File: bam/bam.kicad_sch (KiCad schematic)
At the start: 18 parts, among them J1 battery, Q1 VP3203N3-G, Q2 PN2222A, SW1 pwr, SW2 next, SW3 play/pause, U1 NE555P

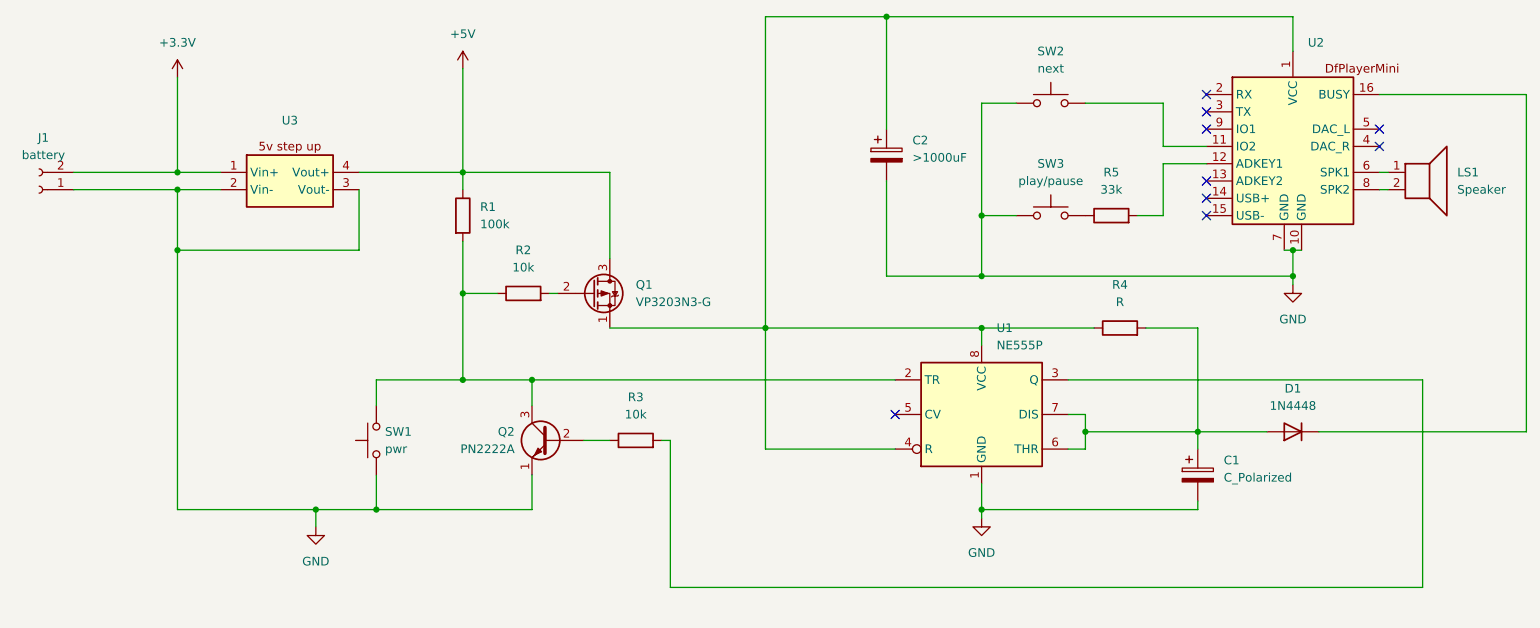
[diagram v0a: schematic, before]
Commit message: true latch
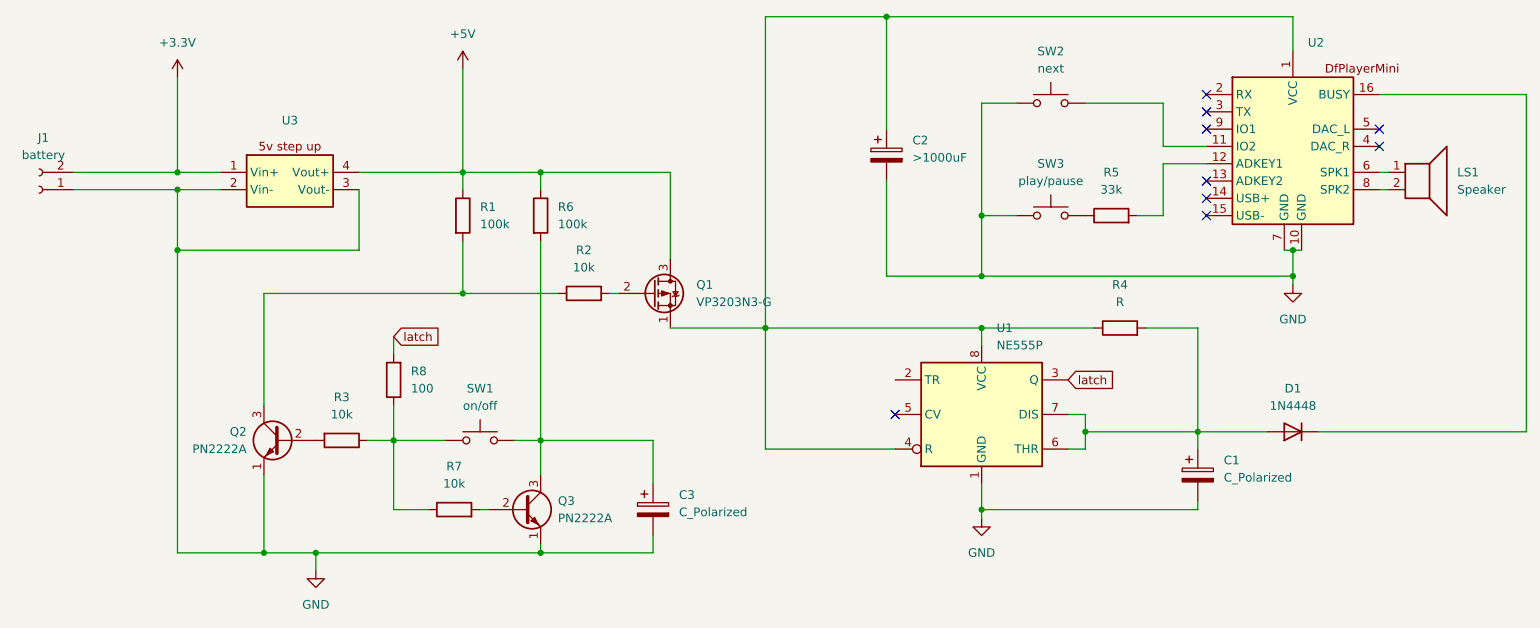
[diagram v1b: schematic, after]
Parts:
- added C3: C_Polarized, symbol Device:C_Polarized
- added Q3: PN2222A, Package_TO_SOT_THT:TO-92_Inline, symbol Transistor_BJT:PN2222A
- added R6: 100k, symbol Device:R
- added R7: 10k, symbol Device:R
- added R8: 100, symbol Device:R
- SW1: value pwr -> on/off
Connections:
- net +5V: now also R6.1
- net GND: now also C3.2, Q3.1 (E); no longer SW1.1
- net at Q2.3 (C), R1.2, R2.1: no longer SW1.2, U1.2 (TR)
- net at R3.1: now also SW1.1, R7.1, R8.1; no longer Q2.2 (B)
- net at R3.2: now also Q2.2 (B); no longer U1.3 (Q)
- new net: Q3.2 (B), R7.2
- new net: C3.1, Q3.3 (C), R6.2, SW1.2
- new net latch: R8.2, U1.3 (Q)
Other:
- moved on the sheet: Q1, Q2, R2
